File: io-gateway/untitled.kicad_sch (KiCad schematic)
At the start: 8 parts, among them J1 1752201, J2 1752201, J3 1752201, J4 Screw_Terminal_01x09, J5 Screw_Terminal_01x09, J6 Screw_Terminal_01x09

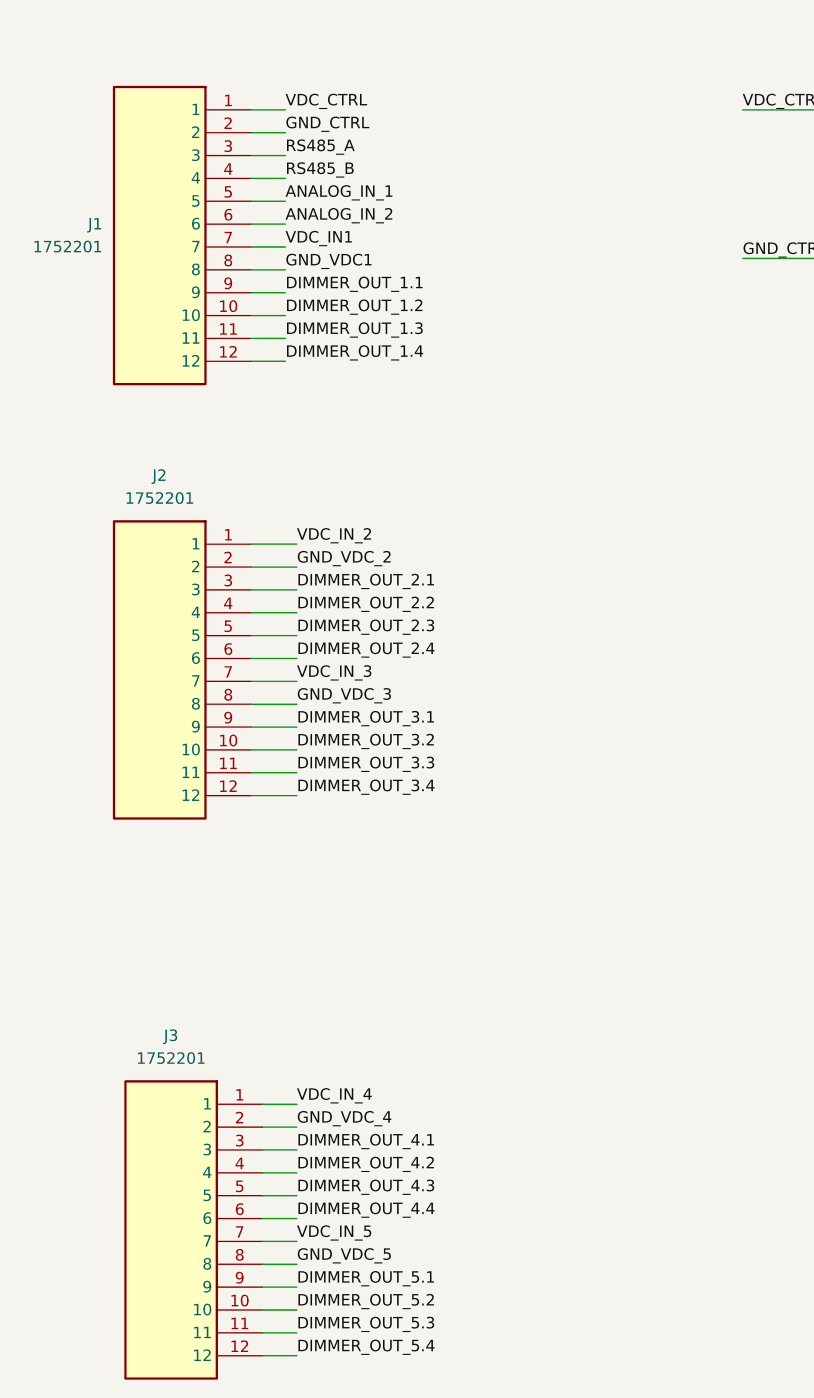
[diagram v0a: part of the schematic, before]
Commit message: update
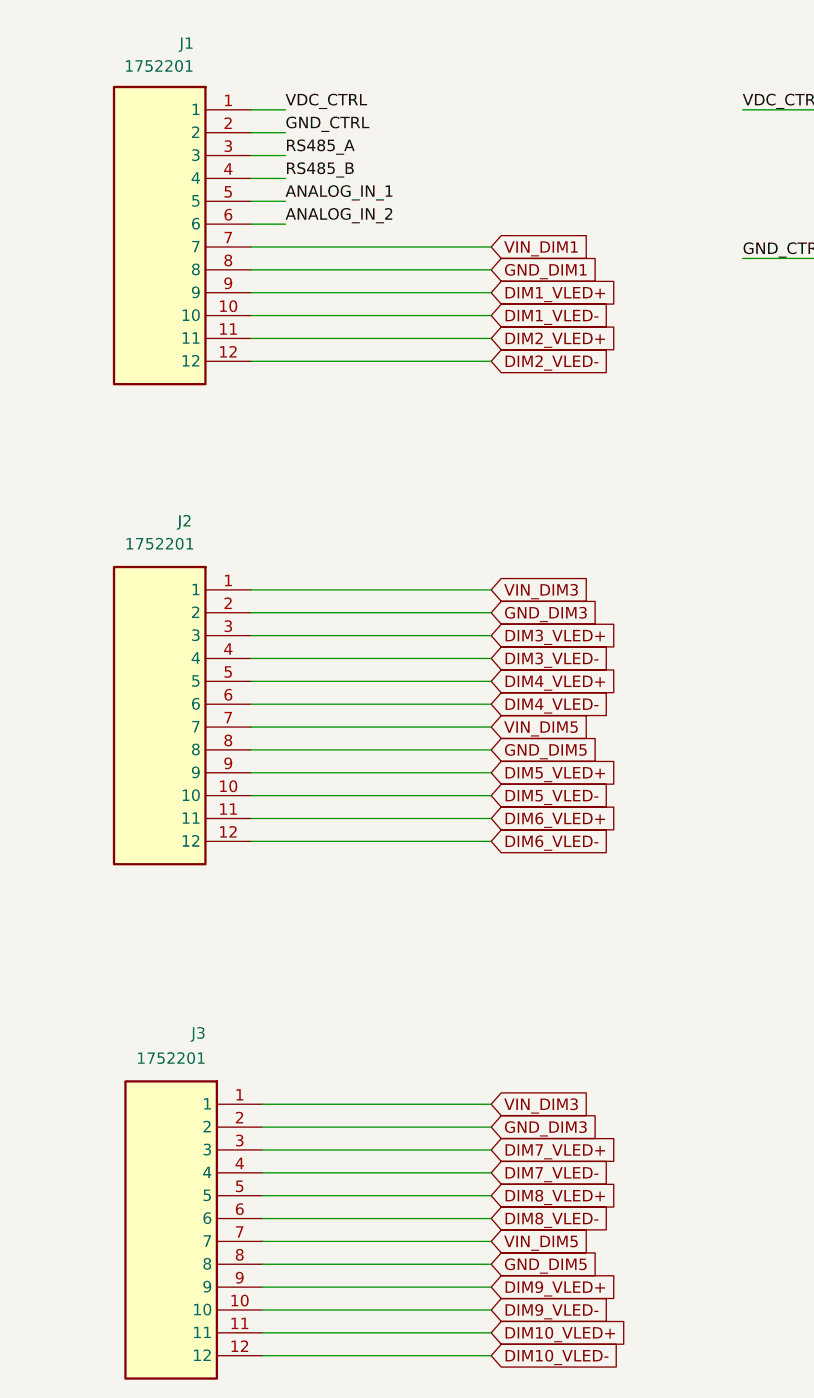
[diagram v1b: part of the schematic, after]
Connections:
- net GND_VDC_4 is gone; now on net GND_DIM3: J3.2
- net GND_VDC_5 is gone; now on net GND_DIM5: J3.8
- net VDC_IN_4 is gone; now on net VIN_DIM3: J3.1
- net VDC_IN_5 is gone; now on net VIN_DIM5: J3.7
- net DIMMER_OUT_1.1 renamed DIM1_VLED+
- net DIMMER_OUT_1.2 renamed DIM1_VLED-
- net DIMMER_OUT_1.3 renamed DIM2_VLED+
- net DIMMER_OUT_1.4 renamed DIM2_VLED-
- net DIMMER_OUT_2.1 renamed DIM3_VLED+
- net DIMMER_OUT_2.2 renamed DIM3_VLED-
- net DIMMER_OUT_2.3 renamed DIM4_VLED+
- net DIMMER_OUT_2.4 renamed DIM4_VLED-
- net DIMMER_OUT_3.1 renamed DIM5_VLED+
- net DIMMER_OUT_3.2 renamed DIM5_VLED-
- net DIMMER_OUT_3.3 renamed DIM6_VLED+
- net DIMMER_OUT_3.4 renamed DIM6_VLED-
- net DIMMER_OUT_4.1 renamed DIM7_VLED+
- net DIMMER_OUT_4.2 renamed DIM7_VLED-
- net DIMMER_OUT_4.3 renamed DIM8_VLED+
- net DIMMER_OUT_4.4 renamed DIM8_VLED-
- net DIMMER_OUT_5.1 renamed DIM9_VLED+
- net DIMMER_OUT_5.2 renamed DIM9_VLED-
- net DIMMER_OUT_5.3 renamed DIM10_VLED+
- net DIMMER_OUT_5.4 renamed DIM10_VLED-
- net GND_VDC1 renamed GND_DIM1
- net GND_VDC_2 renamed GND_DIM3
- net GND_VDC_3 renamed GND_DIM5
- net VDC_IN1 renamed VIN_DIM1
- net VDC_IN_2 renamed VIN_DIM3
- net VDC_IN_3 renamed VIN_DIM5
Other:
- moved on the sheet: J2

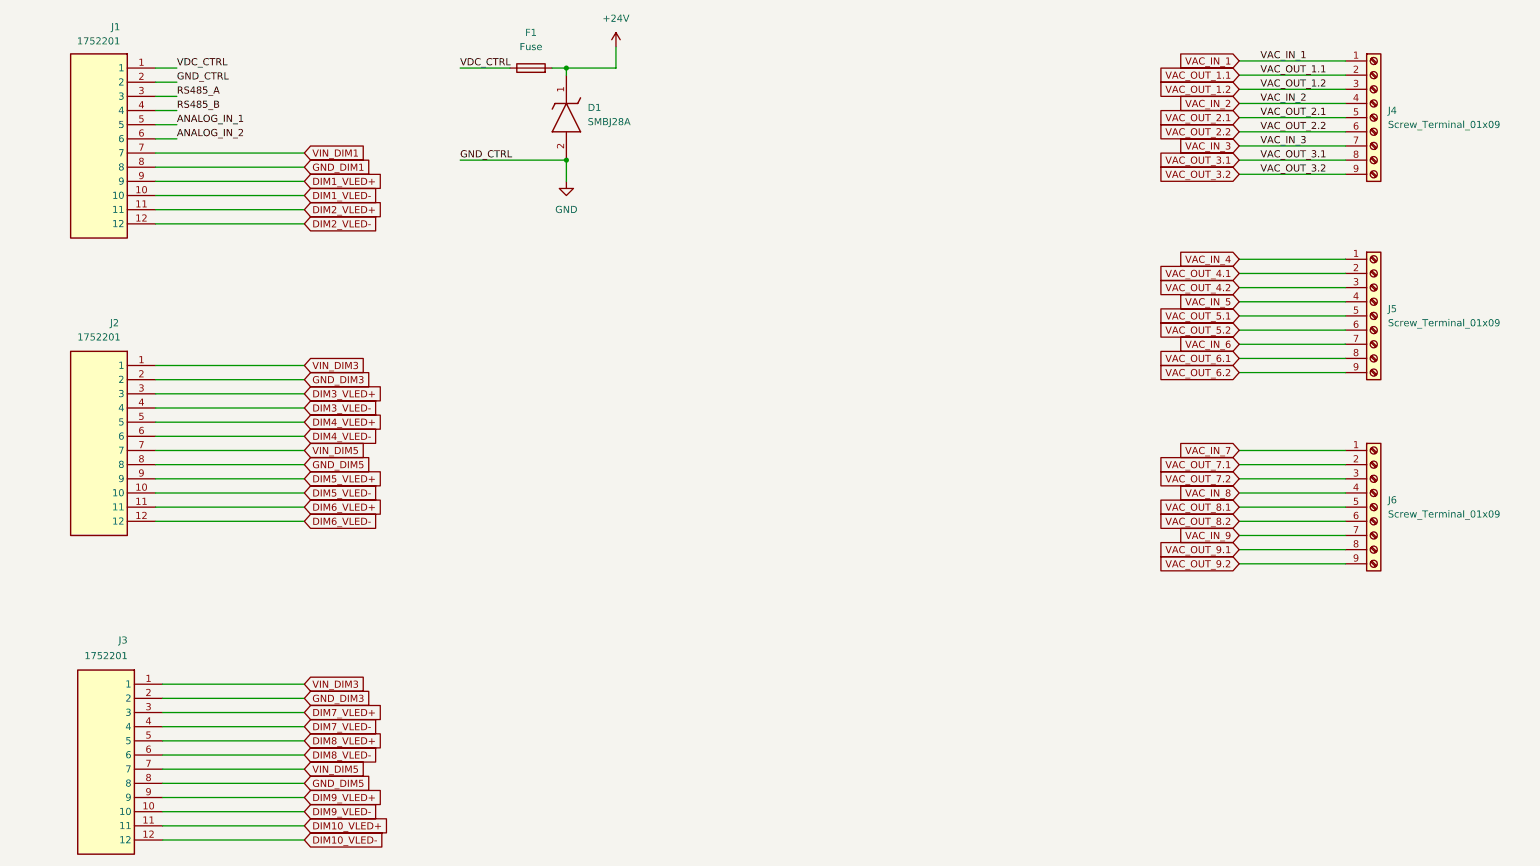
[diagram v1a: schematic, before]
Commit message: layout for first dimmer
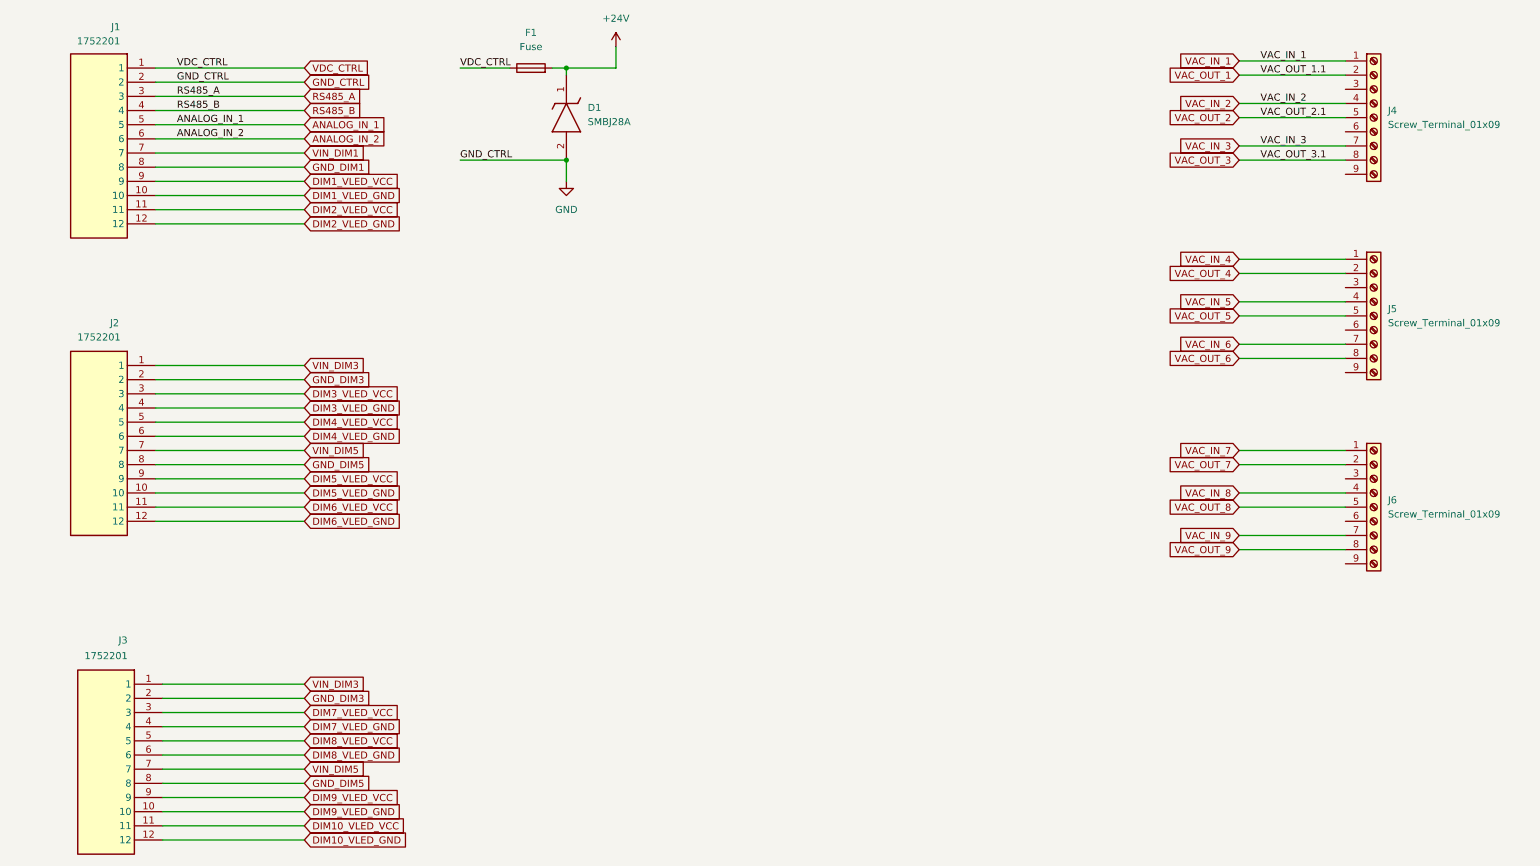
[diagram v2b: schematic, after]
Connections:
- net DIM10_VLED+ renamed DIM10_VLED_VCC
- net DIM10_VLED- renamed DIM10_VLED_GND
- net DIM1_VLED+ renamed DIM1_VLED_VCC
- net DIM1_VLED- renamed DIM1_VLED_GND
- net DIM2_VLED+ renamed DIM2_VLED_VCC
- net DIM2_VLED- renamed DIM2_VLED_GND
- net DIM3_VLED+ renamed DIM3_VLED_VCC
- net DIM3_VLED- renamed DIM3_VLED_GND
- net DIM4_VLED+ renamed DIM4_VLED_VCC
- net DIM4_VLED- renamed DIM4_VLED_GND
- net DIM5_VLED+ renamed DIM5_VLED_VCC
- net DIM5_VLED- renamed DIM5_VLED_GND
- net DIM6_VLED+ renamed DIM6_VLED_VCC
- net DIM6_VLED- renamed DIM6_VLED_GND
- net DIM7_VLED+ renamed DIM7_VLED_VCC
- net DIM7_VLED- renamed DIM7_VLED_GND
- net DIM8_VLED+ renamed DIM8_VLED_VCC
- net DIM8_VLED- renamed DIM8_VLED_GND
- net DIM9_VLED+ renamed DIM9_VLED_VCC
- net DIM9_VLED- renamed DIM9_VLED_GND
- net VAC_OUT_1.1 renamed VAC_OUT_1
- net VAC_OUT_1.2: no longer names the net of J4.3 (Pin_3)
- net VAC_OUT_2.1 renamed VAC_OUT_2
- net VAC_OUT_2.2: no longer names the net of J4.6 (Pin_6)
- net VAC_OUT_3.1 renamed VAC_OUT_3
- net VAC_OUT_3.2: no longer names the net of J4.9 (Pin_9)
- net VAC_OUT_4.1 renamed VAC_OUT_4
- net VAC_OUT_4.2: no longer names the net of J5.3 (Pin_3)
- net VAC_OUT_5.1 renamed VAC_OUT_5
- net VAC_OUT_5.2: no longer names the net of J5.6 (Pin_6)
- net VAC_OUT_6.1 renamed VAC_OUT_6
- net VAC_OUT_6.2: no longer names the net of J5.9 (Pin_9)
- net VAC_OUT_7.1 renamed VAC_OUT_7
- net VAC_OUT_7.2: no longer names the net of J6.3 (Pin_3)
- net VAC_OUT_8.1 renamed VAC_OUT_8
- net VAC_OUT_8.2: no longer names the net of J6.6 (Pin_6)
- net VAC_OUT_9.1 renamed VAC_OUT_9
- net VAC_OUT_9.2: no longer names the net of J6.9 (Pin_9)
